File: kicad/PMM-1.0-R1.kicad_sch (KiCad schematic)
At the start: 29 parts, among them U1 TLV75733PDBV, U11 TPS22917DBV, U2 BQ25895RTW, U4 BQ27441-G1, U6 TPS61089, U9 STM32C031C4T6

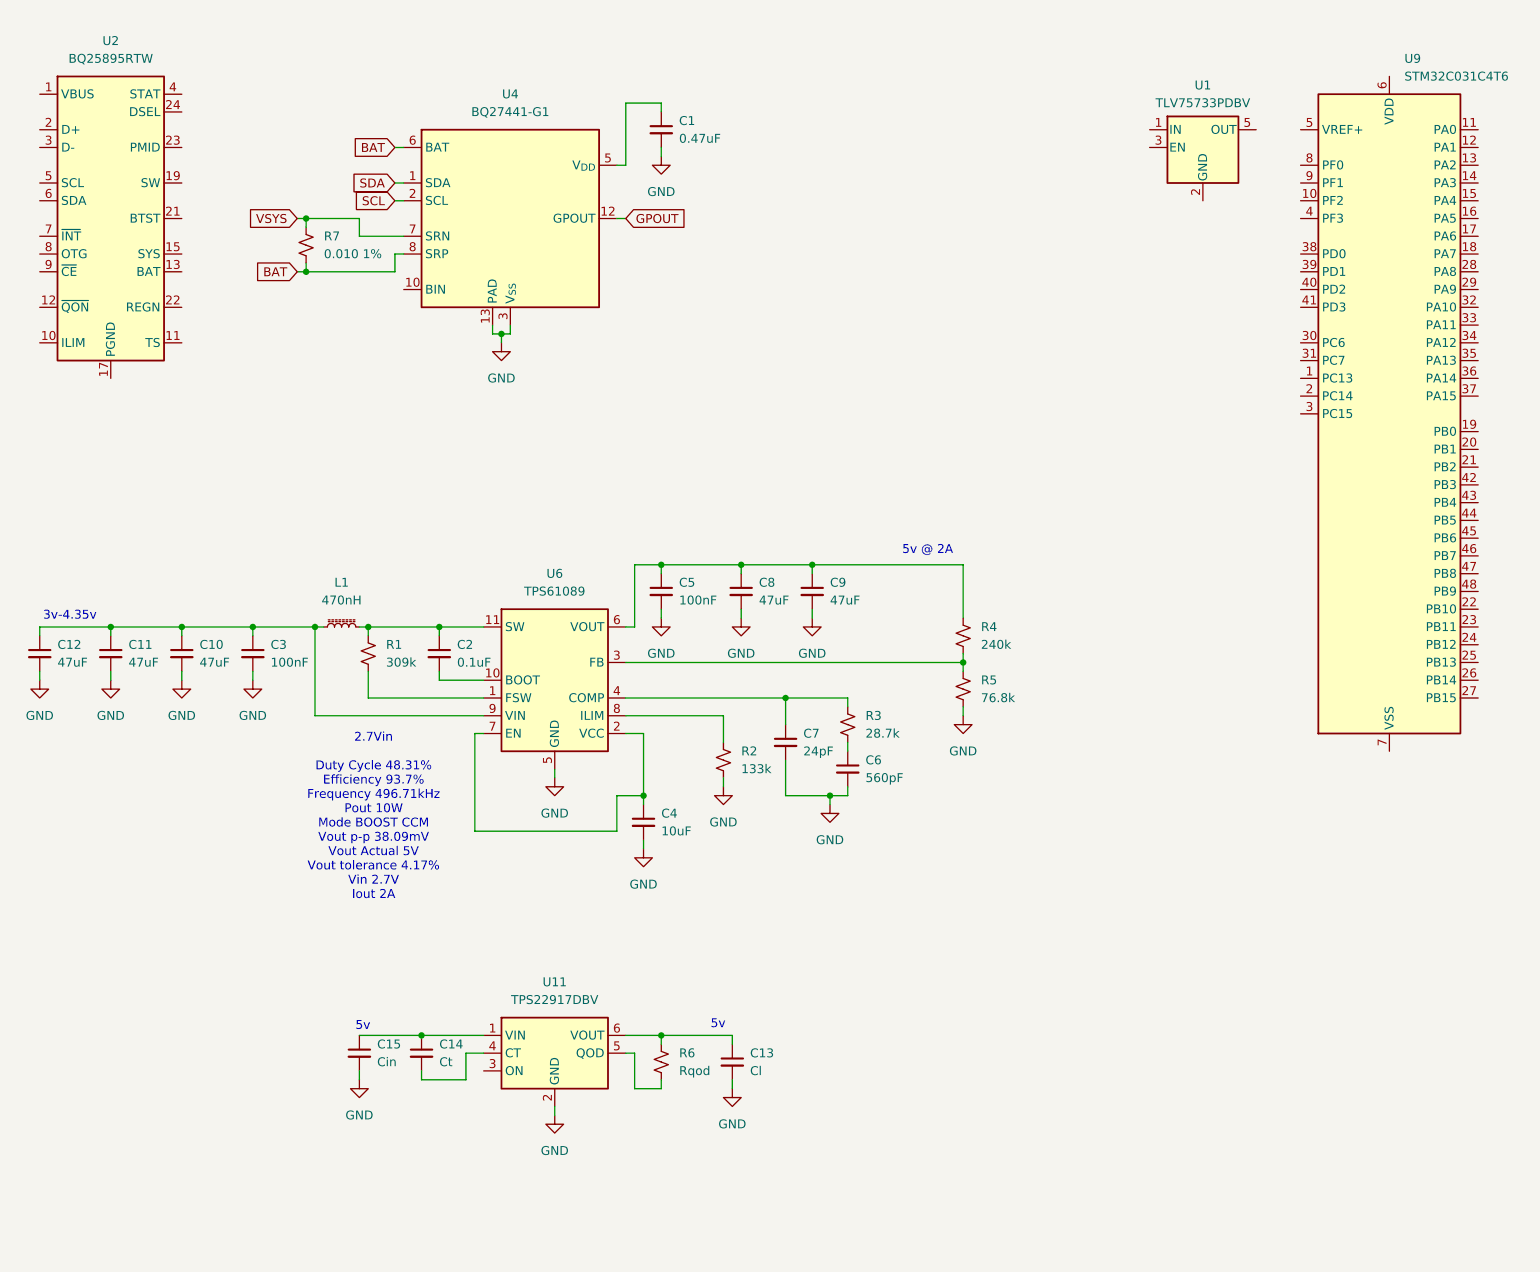
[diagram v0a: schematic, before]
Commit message: updates
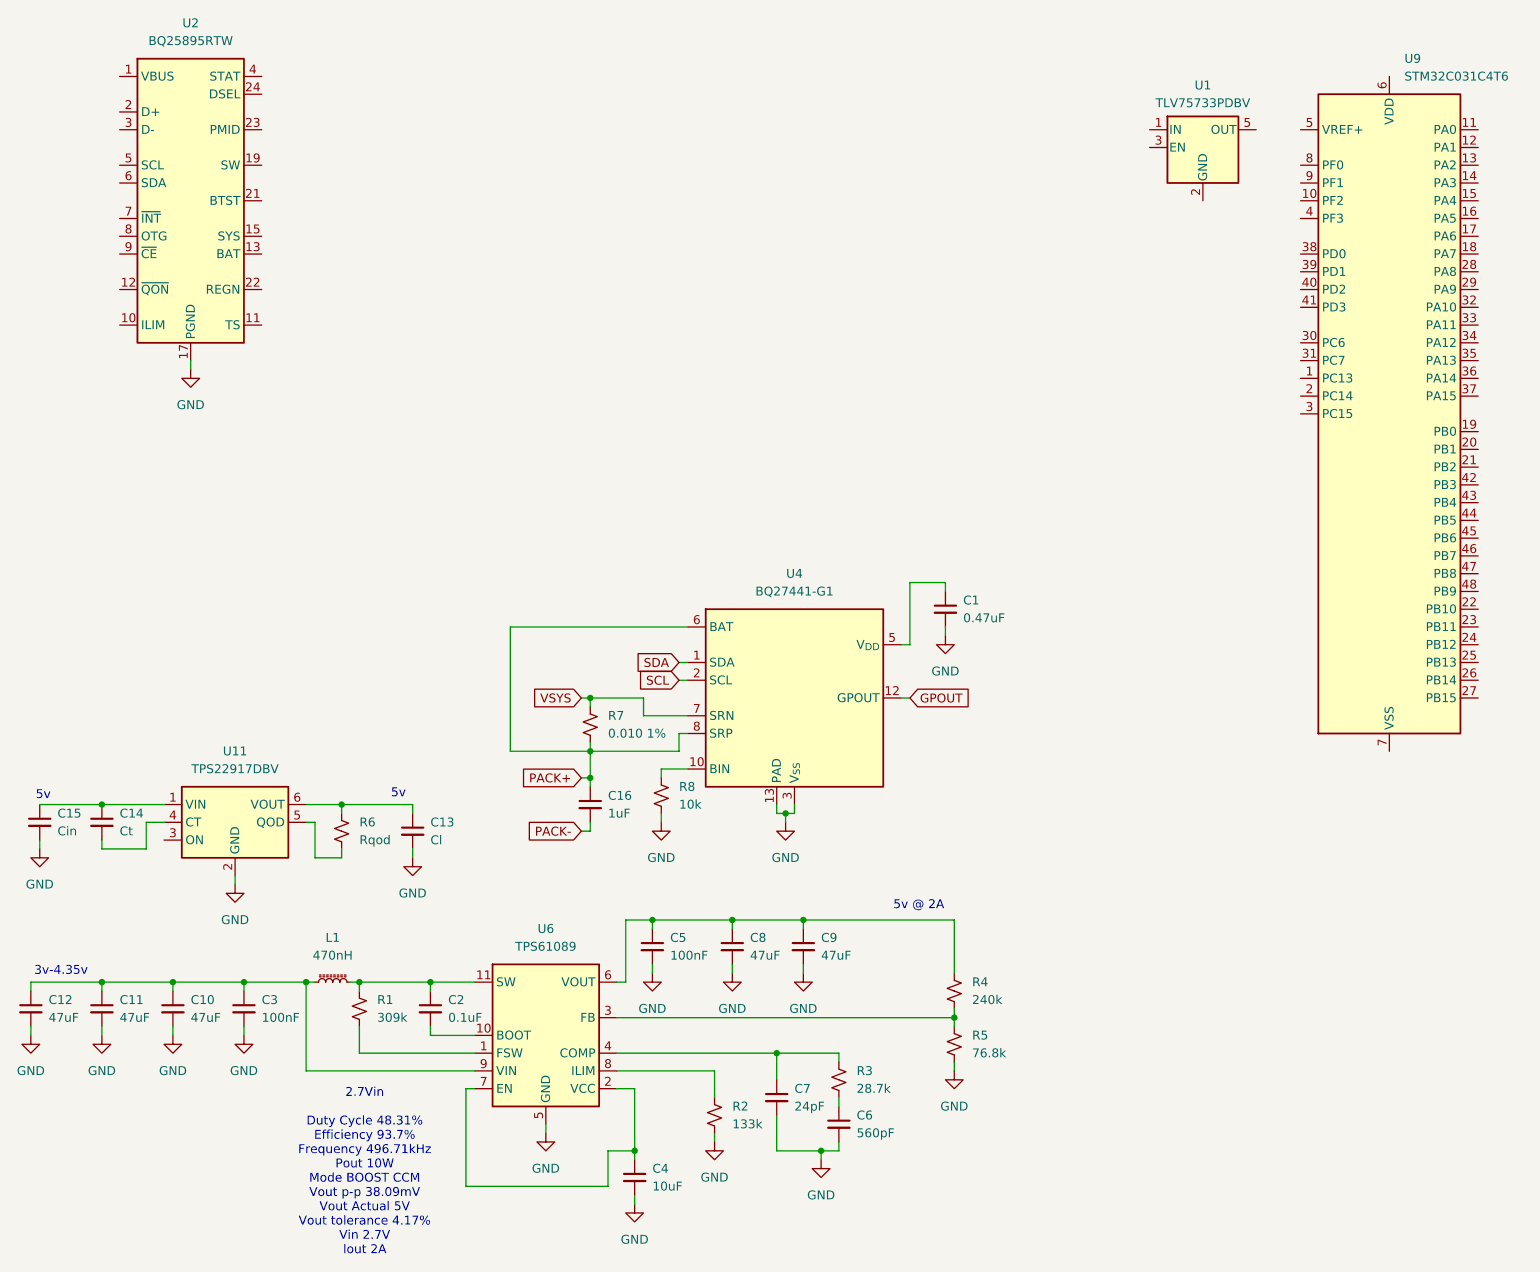
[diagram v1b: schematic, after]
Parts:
- added C16: 1uF, symbol Device:C_Small
- added R8: 10k, symbol Device:R_Small_US
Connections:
- net GND: now also U2.17 (PGND), U2.18 (PGND), U2.25 (PGND), R8.2
- net at U4.10 (BIN): now also R8.1
- net BAT renamed PACK+
- net PACK+: now also C16.1
- new net PACK-: C16.2
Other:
- moved on the sheet: C1, C10, C11, C12, C13, C14, C15, C2, C3, C4, C5, C6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
